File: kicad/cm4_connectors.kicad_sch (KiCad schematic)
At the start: 9 parts, among them J11 2541WV-2X12P, J12 Header-Male-2.54_2x3, J13 Header-Male-2.54_1x3, J2 Header-Male-2.54_2x3, U15 74LVC1G07SE-7

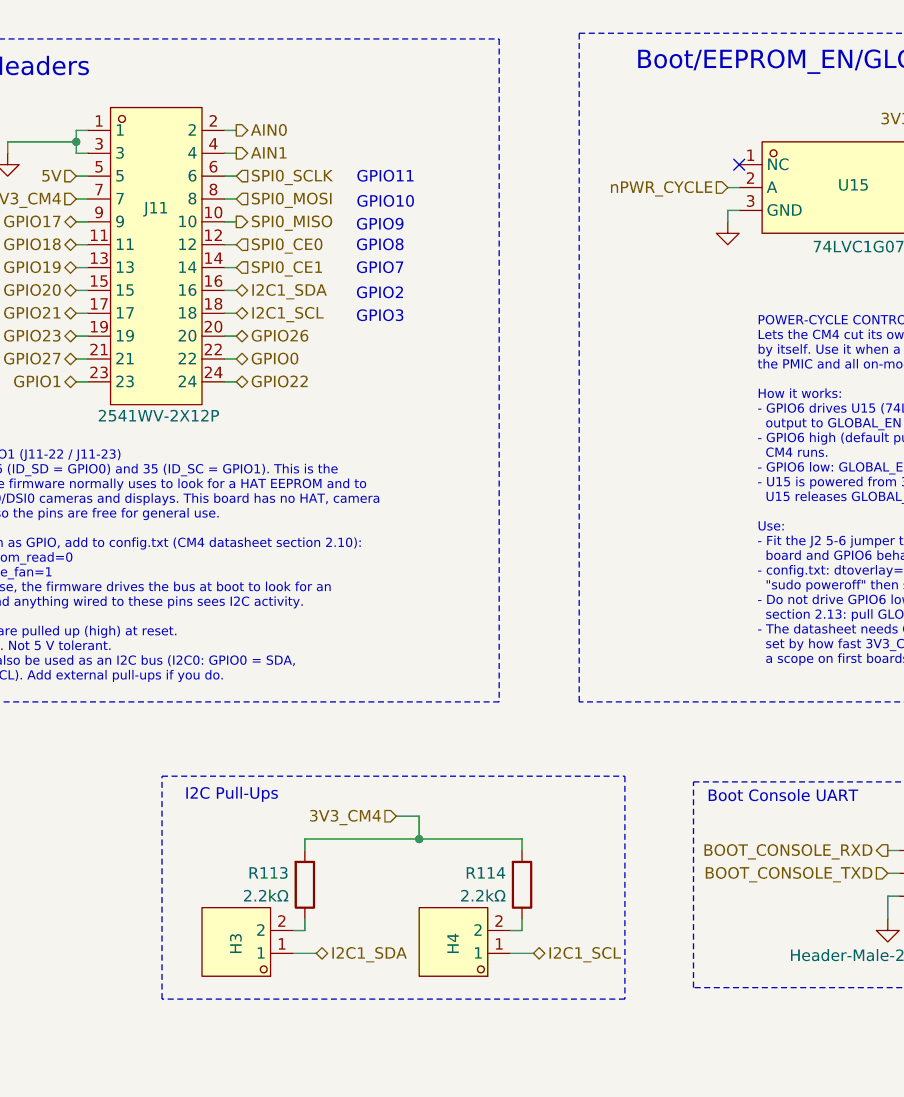
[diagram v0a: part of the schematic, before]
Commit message: schematic cleanup
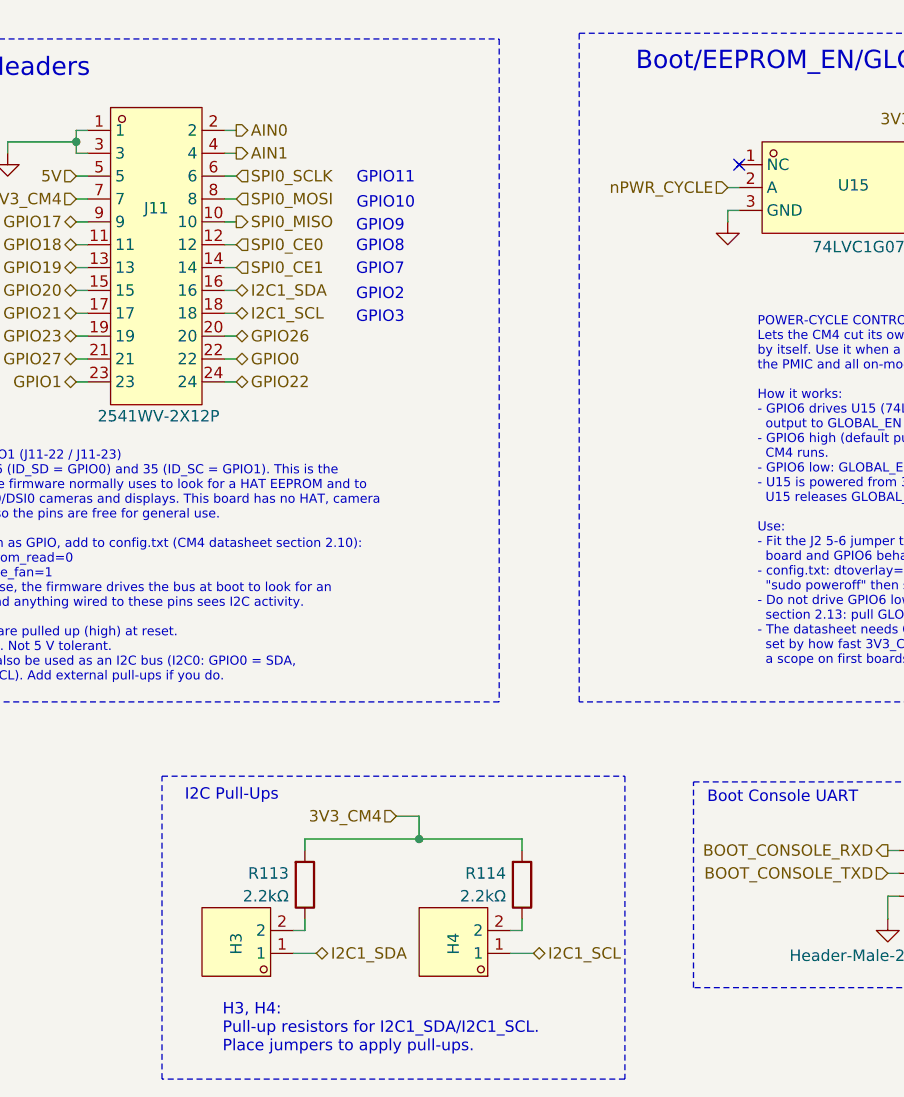
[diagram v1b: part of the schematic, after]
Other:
- note added: "H3, H4: Pull-up resistors for I2C1_SDA/I2C1_SCL. Place jumpers to apply pull-ups."
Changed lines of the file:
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@@
 	(rectangle
 		(start 80.645 130.175)
-		(end 132.08 154.94)
+		(end 132.08 163.83)
 		(stroke
 			(width 0)
@@
 		)
 	)
+	(text "H3, H4:\nPull-up resistors for I2C1_SDA/I2C1_SCL.\nPlace jumpers to apply pull-ups."
+		(exclude_from_sim no)
+		(at 87.376 158.242 0)
+		(effects
+			(font
+				(size 1.27 1.27)
+			)
+			(justify left)
+		)
+	)

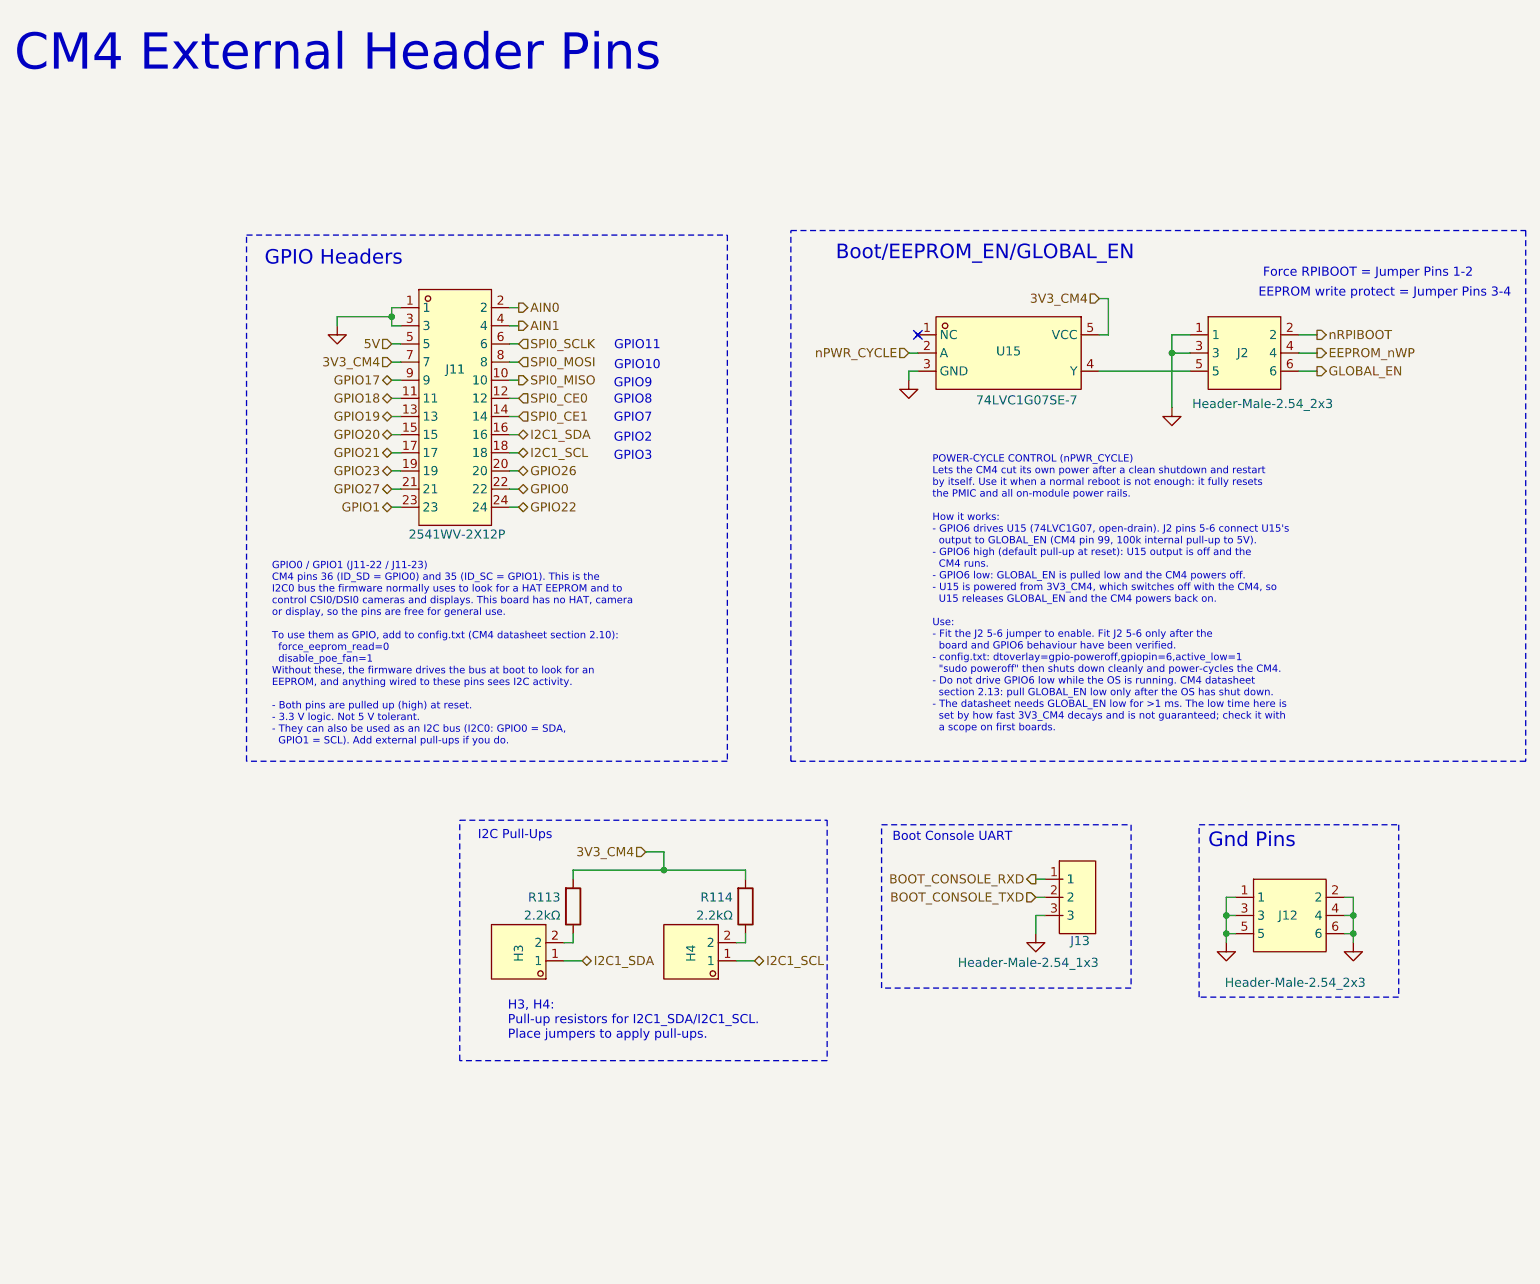
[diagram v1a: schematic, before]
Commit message: Still refining
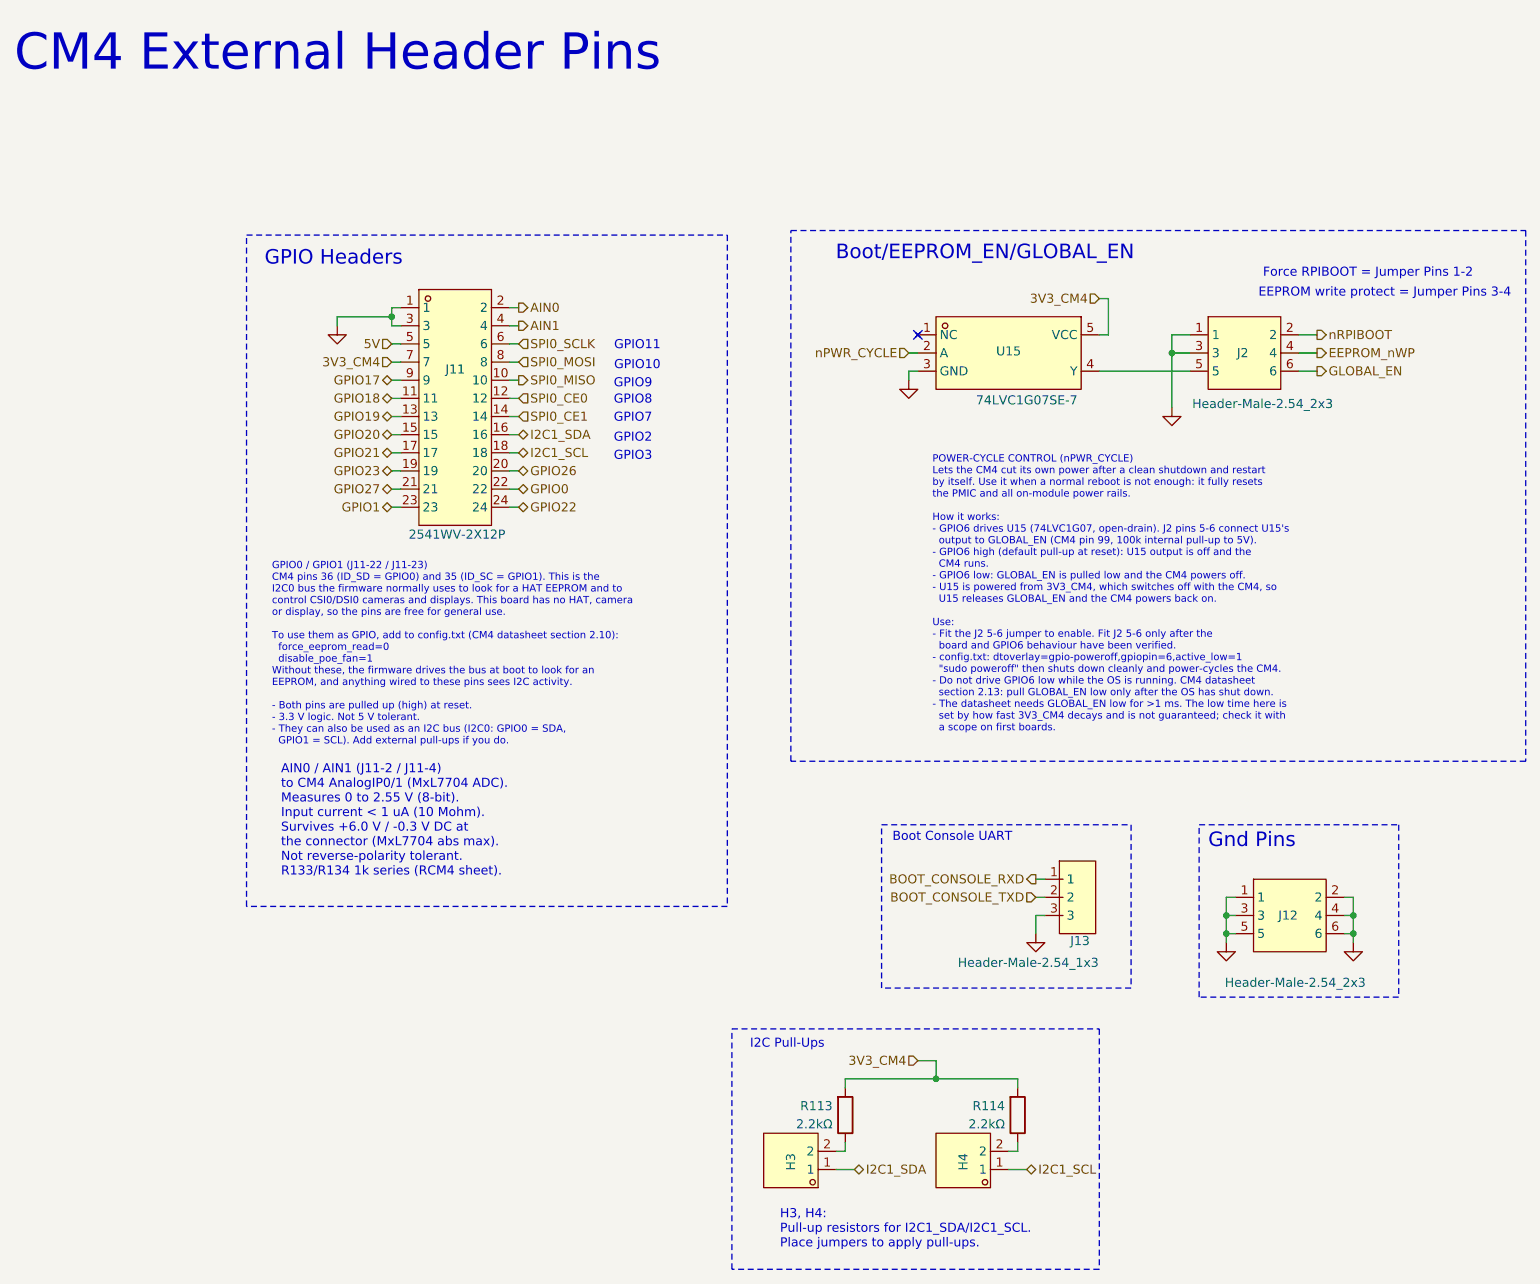
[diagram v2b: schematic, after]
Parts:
- H3, H4: Pkg Type (none) -> THT Pin header 1x2 P2.54
- J11: Pkg Type (none) -> THT Pin header 2x12 P2.54
- J12, J2: Pkg Type (none) -> THT Pin header 2x3 P2.54
- J13: Pkg Type (none) -> THT Pin header 1x3 P2.54
- R113, R114: Pkg Type (none) -> SMD 0402
- U15: Pkg Type (none) -> SMD SOT-353 (SC-88A)
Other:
- note added: "AIN0 / AIN1 (J11-2 / J11-4) to CM4 AnalogIP0/1 (MxL7704 ADC). Measures 0 to 2.55 V (8-bit). Input current < 1 uA (10 Mohm). Survives +6.0 V / -0.3 V DC at the connector (MxL7704 abs max). Not reverse-polarity tolerant. R133/R134 1k series (RCM4 sheet)."
- moved on the sheet: H3, H4, R113, R114
